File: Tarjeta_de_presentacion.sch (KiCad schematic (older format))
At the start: 23 parts, among them J1 Batería, J2 Conn_01x06, J3 Directa, J4 Pines analógicos, J5 Pines Digitales, J6 SPI, J7 I2C, J8 Fuente, SW1 Reset, U1 ATMEGA328P-AU, Y1 Crystal

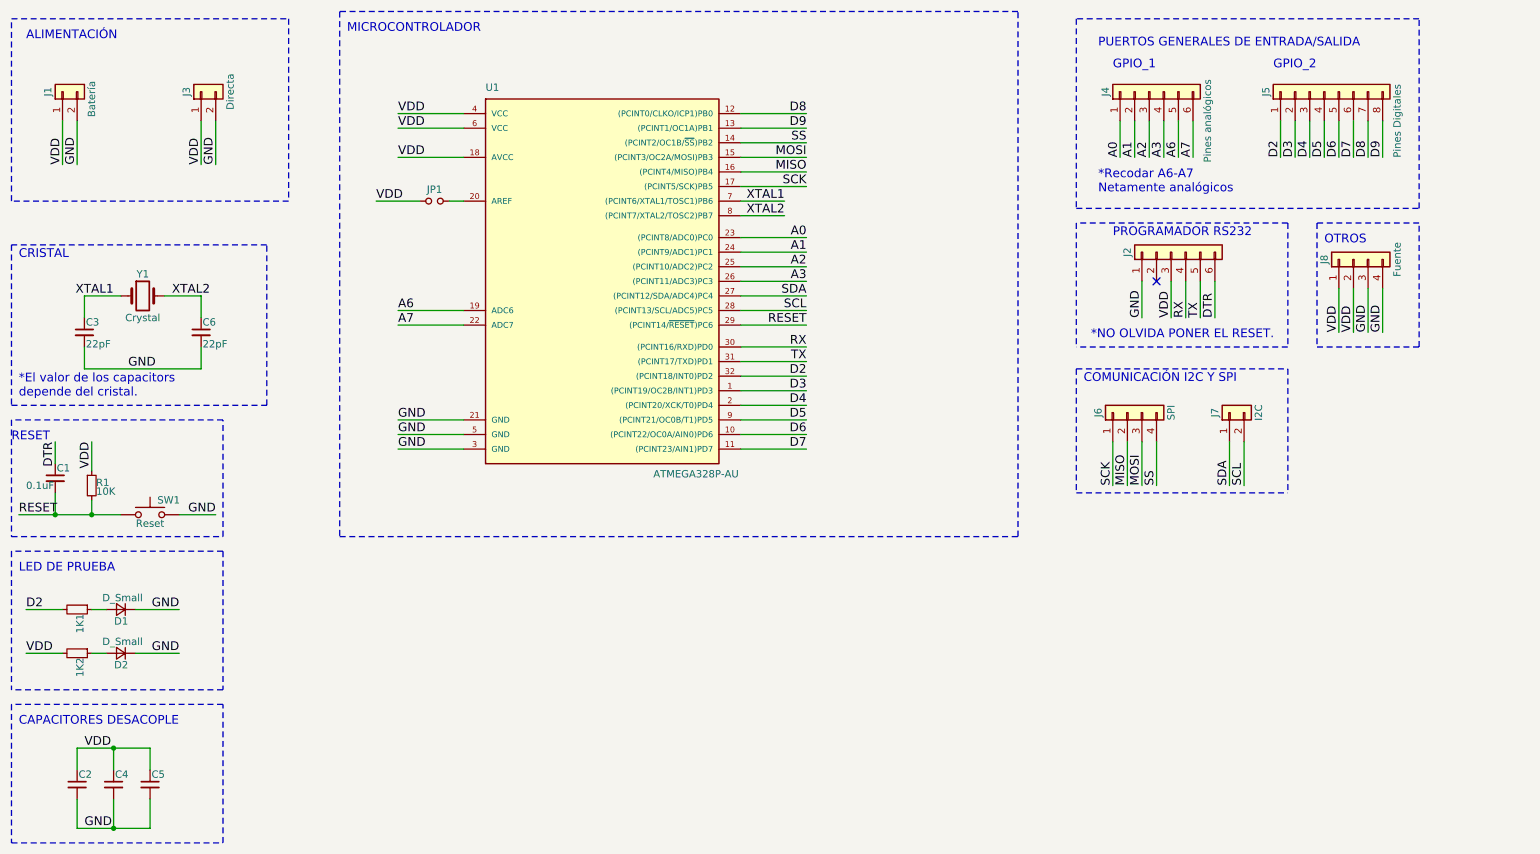
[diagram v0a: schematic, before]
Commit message: /
//
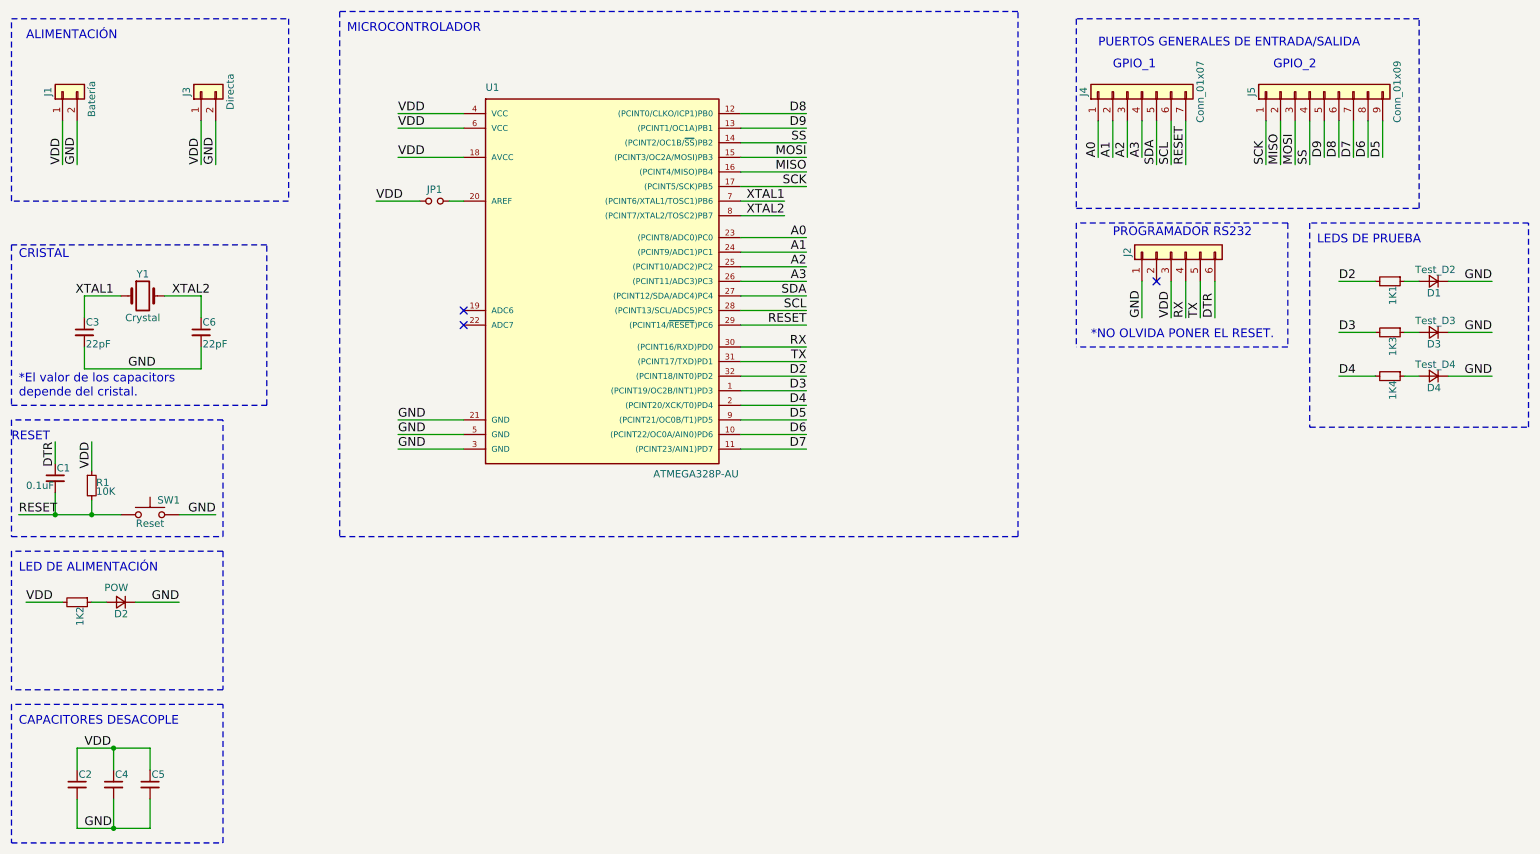
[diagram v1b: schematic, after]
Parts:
- removed J4: Pines analógicos, Pin_Headers:Pin_Header_Straight_1x06_Pitch2.54mm, symbol Conn_01x06
- removed J5: Pines Digitales, Pin_Headers:Pin_Header_Straight_1x08_Pitch2.54mm, symbol Conn_01x08
- removed J6: SPI, Pin_Headers:Pin_Header_Straight_1x04_Pitch2.54mm, symbol Conn_01x04
- removed J7: I2C, Pin_Headers:Pin_Header_Straight_1x02_Pitch2.54mm, symbol Conn_01x02
- removed J8: Fuente, Pin_Headers:Pin_Header_Straight_1x04_Pitch2.54mm, symbol Conn_01x04
- added 1K3, 1K4: R_Small, Resistors_SMD:R_0805_HandSoldering, symbol R_Small
- added D3: Test_D3, Diodes_SMD:D_0805, symbol D_Small
- added D4: Test_D4, Diodes_SMD:D_0805, symbol D_Small
- added J4: Conn_01x07, Pin_Headers:Pin_Header_Straight_1x07_Pitch2.54mm, symbol Conn_01x07
- added J5: Conn_01x09, Pin_Headers:Pin_Header_Straight_1x09_Pitch2.54mm, symbol Conn_01x09
- D1: value D_Small -> Test_D2
- D2: value D_Small -> POW
- J1: footprint Pin_Headers:Pin_Header_Straight_1x02_Pitch2.54mm -> Librerias_FootPrints:Holder_Battery
- SW1: footprint (none) -> Librerias_FootPrints:Boton_Single
- Y1: footprint (none) -> Crystals:Crystal_HC49-4H_Vertical
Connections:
- net A0: now also J4.1 (Pin_1)
- net A1: now also J4.2 (Pin_2)
- net A2: now also J4.3 (Pin_3)
- net A3: now also J4.4 (Pin_4)
- net D3: now also 1K3.2
- net D4: now also 1K4.2
- net D5: now also J5.9 (Pin_9)
- net D6: now also J5.8 (Pin_8)
- net D7: now also J5.7 (Pin_7)
- net D8: now also J5.6 (Pin_6)
- net D9: now also J5.5 (Pin_5)
- net GND: now also D3.1 (K), D4.1 (K)
- net MISO: now also J5.2 (Pin_2)
- net MOSI: now also J5.3 (Pin_3)
- net RESET: now also J4.7 (Pin_7)
- net SCK: now also J5.1 (Pin_1)
- net SCL: now also J4.6 (Pin_6)
- net SDA: now also J4.5 (Pin_5)
- net SS: now also J5.4 (Pin_4)
- net A6: no longer names the net of U1.19 (ADC6)
- net A7: no longer names the net of U1.22 (ADC7)
- new net: 1K3.1, D3.2 (A)
- new net: 1K4.1, D4.2 (A)
- no-connect marks 1 -> 3
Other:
- note added: "LED DE ALIMENTACIÓN"
- note added: "LEDS DE PRUEBA"
- note removed: "*Recodar A6-A7\nNetamente analógicos"
- note removed: "COMUNICACIÓN I2C Y SPI"
- note removed: "LED DE PRUEBA"
- note removed: "OTROS"
- moved on the sheet: 1K1, 1K2, D1, D2
